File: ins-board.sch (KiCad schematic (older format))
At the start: 80 parts, among them Q1 FDN306P, U2 STM32F415RGT6, U4 MAX3051, U6 LT1761-3.3, U7 LT1965, X1 CRYSTAL 16MHz 10ppm

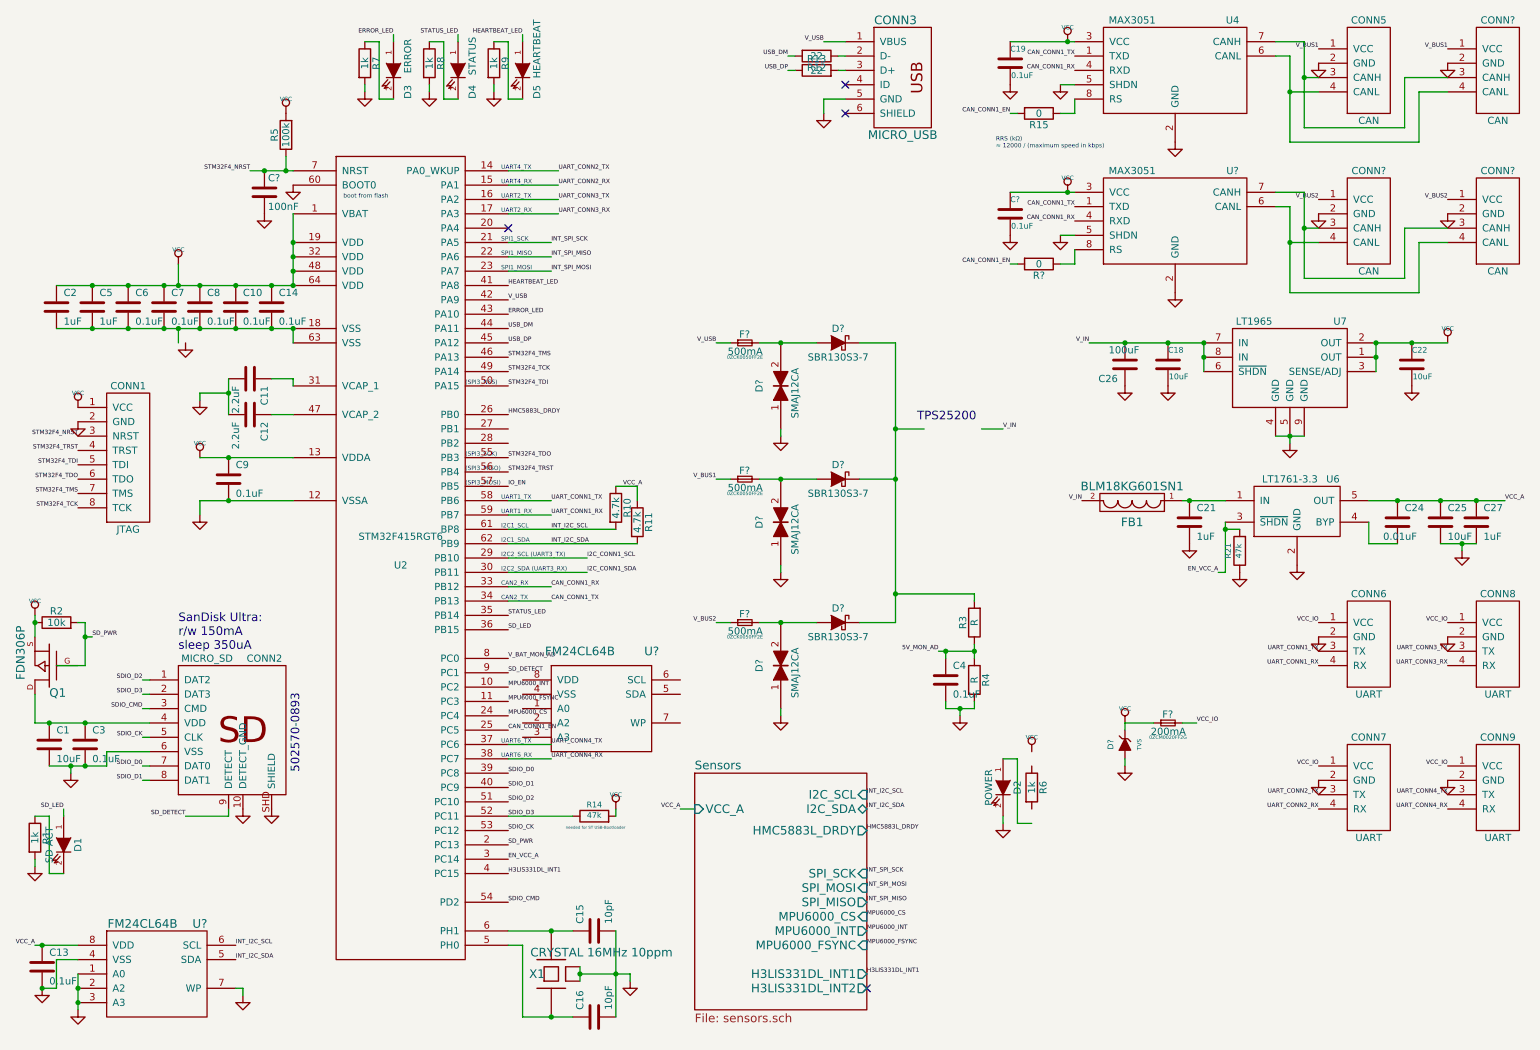
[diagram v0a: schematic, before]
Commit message: schematic organization
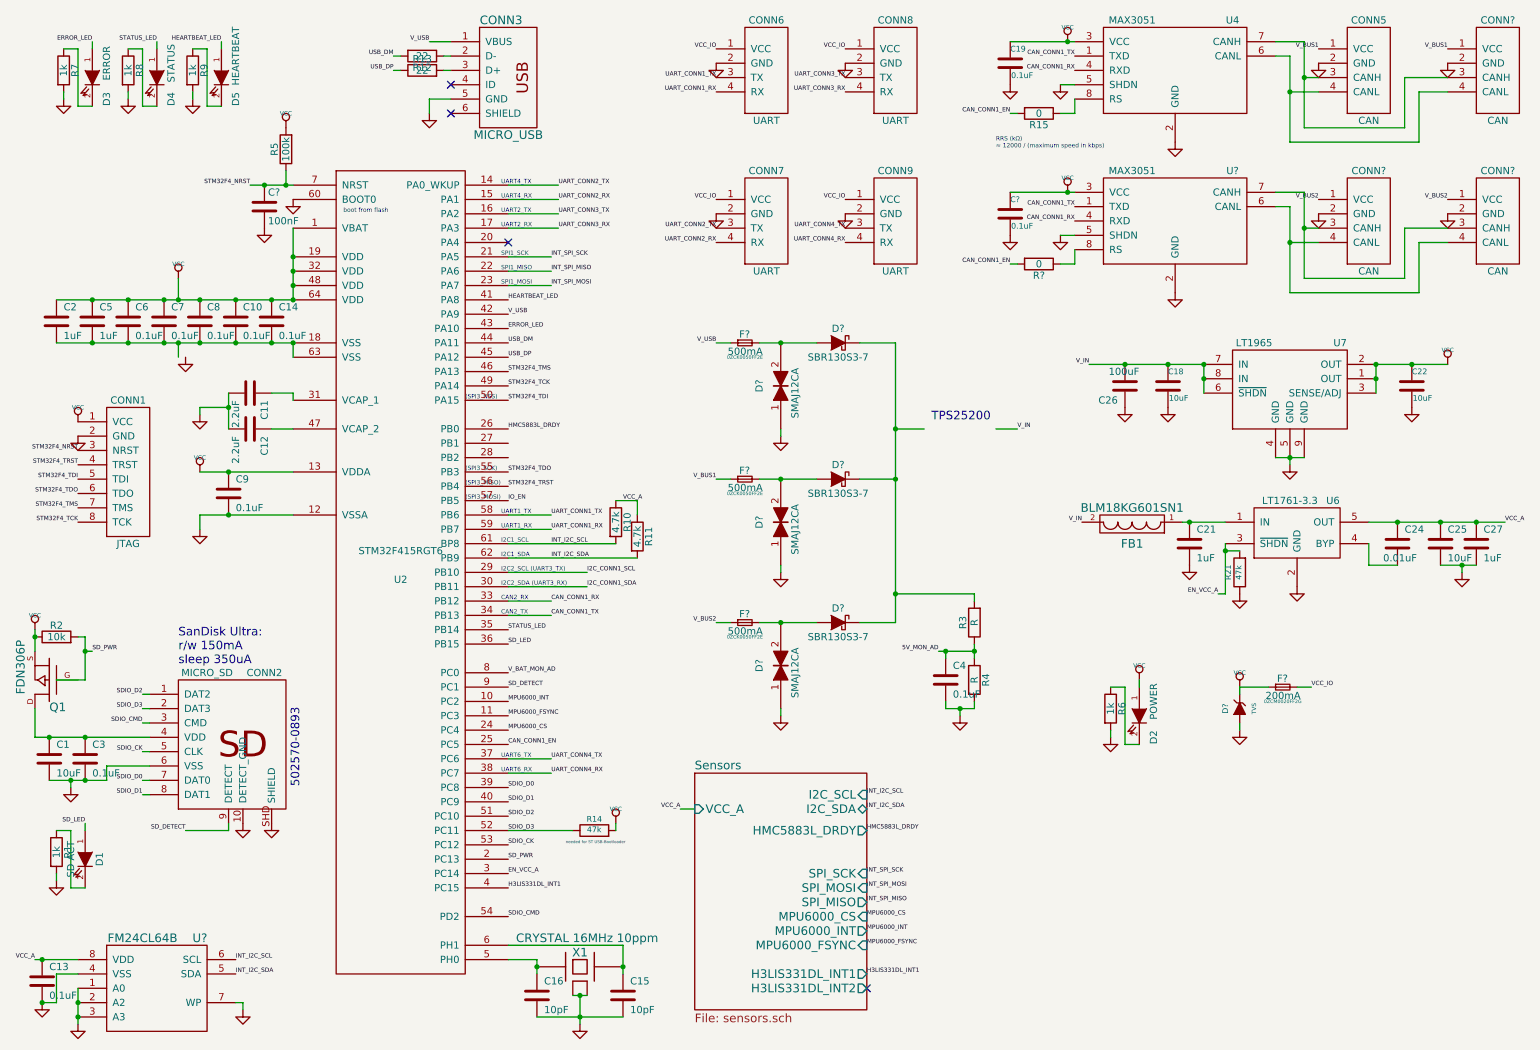
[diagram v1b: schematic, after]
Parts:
- removed U?: FM24CL64B, symbol FM24CL64B
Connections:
- net GND: now also R6.2; no longer D2.2 (K)
- net VCC: now also D2.1 (A)
- net at R6.1: now also D2.2 (K)
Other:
- moved on the sheet: C1, C10, C11, C12, C13, C14, C15, C16, C18, C2, C21, C22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
